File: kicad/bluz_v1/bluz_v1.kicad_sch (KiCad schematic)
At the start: 59 parts, among them J1 USB_B_Micro, J11 Conn, J12 BTAnt, J2 Conn, J3 Conn, J4 Conn, J5 Conn, J6 Conn, J7 Conn, J8 Conn, M1 VibroMotor, Q1 RUM002N05, Q2 RUM002N05, SW1 SW_DPDT_x2, U1 MCP73831, U2 MCP1700, U3 TLV3201AIDCK, Y1 NX2016SA-32MHz

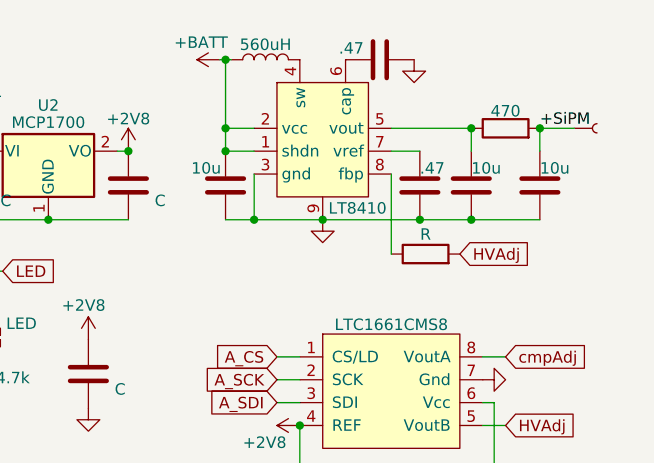
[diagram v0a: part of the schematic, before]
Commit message: удалено:       kicad/bluz_v1/bluz_v1-backups/bluz_v1-2024-04-19_190122.zip 	удалено:       kicad/bluz_v1/bluz_v1-backups/bluz_v1-2024-04-22_153028.zip 	удалено:       kicad/bluz_v1/bluz_v1-backups/bluz_v1-2024-04-26_142701.zip 	удалено:       kicad/bluz_v1/bluz_v1-backups/bluz_v1-2024-05-03_144119.zip 	удалено:       kicad/bluz_v1/bluz_v1-backups/bluz_v1-2024-05-03_145331.zip 	изменено:      kicad/bluz_v1/bluz_v1.kicad_pcb 	изменено:      kicad/bluz_v1/bluz_v1.kicad_sch 	изменено:      kicad/bluz_v1/fp-info-cache
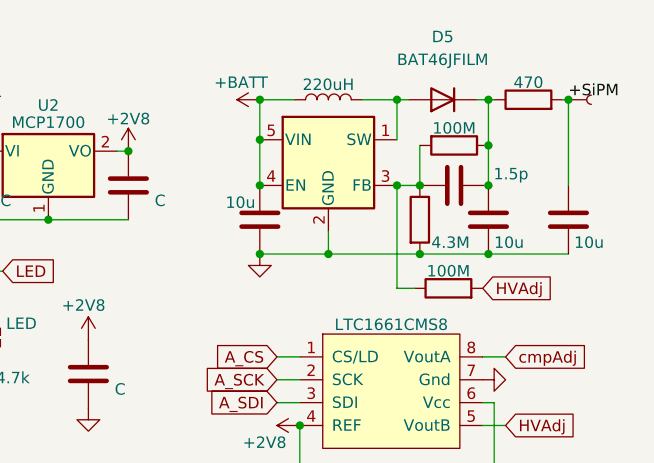
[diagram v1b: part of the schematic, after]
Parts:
- removed C17: .47, Capacitor_SMD:C_0402_1005Metric, symbol Device:C
- removed C18: 10u, Capacitor_SMD:C_1206_3216Metric, symbol Device:C
- removed D5: LT8410, Package_DFN_QFN:DFN-8-1EP_2x2mm_P0.45mm_EP0.64x1.38mm, symbol My-Library:LT8410
- added C9: 1.5p, Capacitor_SMD:C_0402_1005Metric, symbol Device:C
- added D5: BAT46JFILM, Diode_SMD:D_SOD-323, symbol Device:D
- added R15: 4.3M, Resistor_SMD:R_0402_1005Metric, symbol Device:R
- added R16: 100M, Resistor_SMD:R_0603_1608Metric, symbol Device:R
- added U4: AP3015KTR, Package_TO_SOT_SMD:SOT-23-5, symbol My_Library:AP3015KTR
- BZ1: footprint lib:Buzzer5x5 -> MyLibrary:Buzzer55x55
- C16: value .47 -> 10u; footprint Capacitor_SMD:C_0402_1005Metric -> Capacitor_SMD:C_0805_2012Metric
- C19: footprint Capacitor_SMD:C_1206_3216Metric -> Capacitor_SMD:C_0805_2012Metric
- L2: value 560uH -> 220uH
- R13: value R -> 100M
- U2: footprint Package_TO_SOT_SMD:SOT-23 -> Package_TO_SOT_SMD:SOT-23-3
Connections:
- net +BATT: now also U4.4 (EN), U4.5 (VIN)
- net GND: now also C16.1, R15.2, U4.2 (GND); no longer C16.2
- net at L2.2: now also D5.2 (A), U4.1 (SW)
- net at R14.1: now also C16.2, C9.1, D5.1 (K), R16.1
- net at R13.1: now also C9.2, R15.1, R16.2, U4.3 (FB)
